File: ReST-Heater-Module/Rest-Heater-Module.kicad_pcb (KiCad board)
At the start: 2 copper layers, 24.5 x 29.5 mm, 35 parts

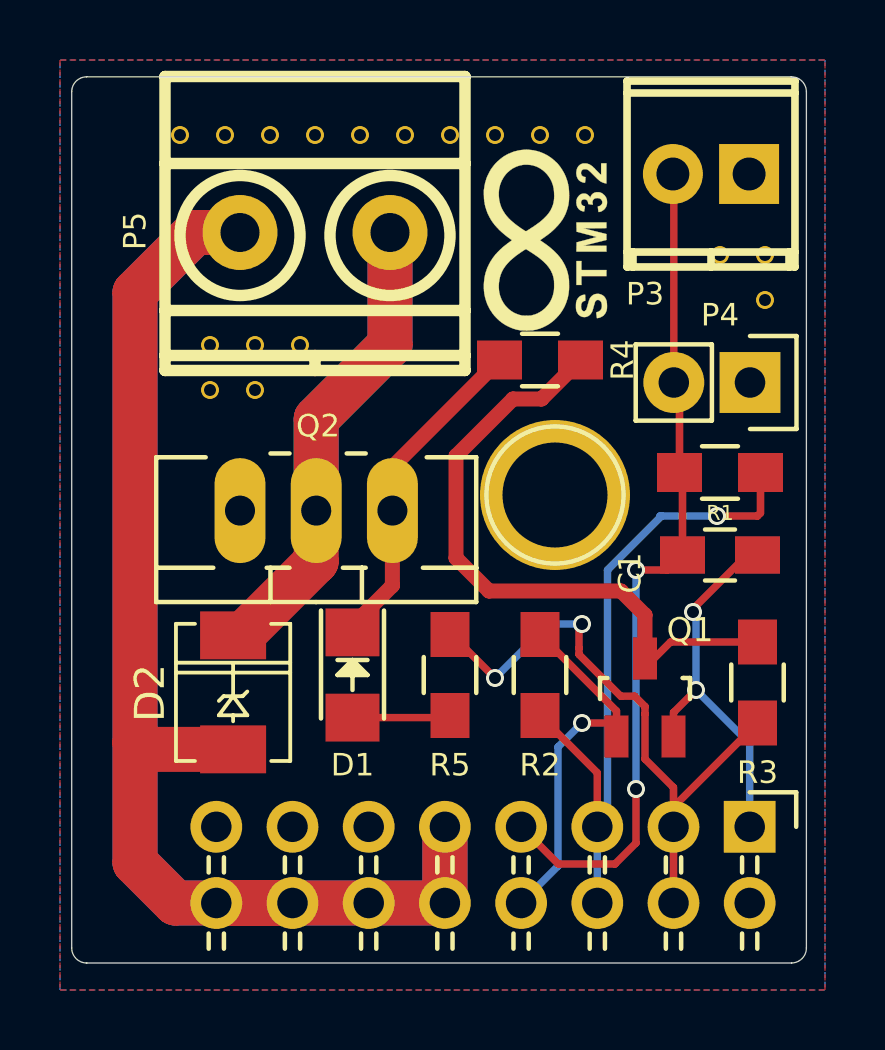
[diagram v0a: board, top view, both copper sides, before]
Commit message: Final release
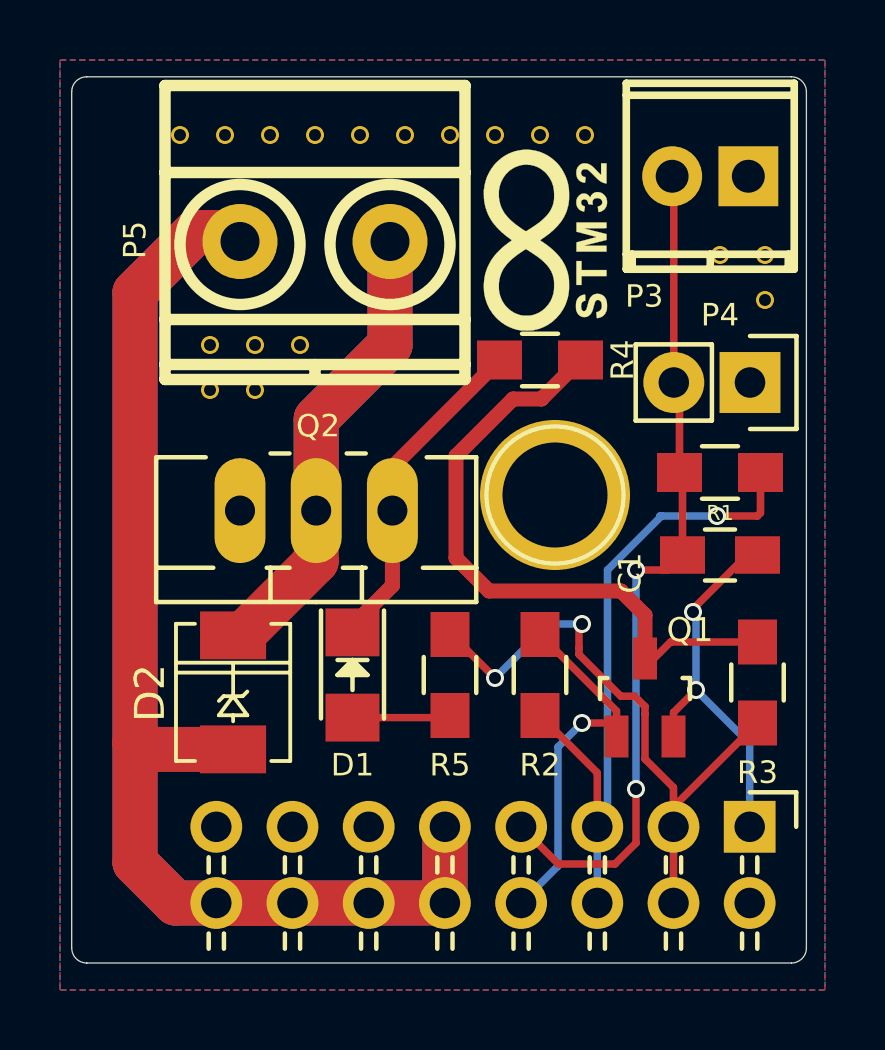
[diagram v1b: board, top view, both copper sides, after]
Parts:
- moved P5 0.30 mm to (141.0, 110.5)
- moved P3 0.08 mm to (154.2, 108.4)
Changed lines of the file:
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@@
     (links 52)
     (no_connects 0)
-    (area 132.5 102.875 159.575 143.485001)
+    (area 132.5 102.875 159.575 135.500001)
     (thickness 1.6)
     (drawings 9)
@@
     (visible_elements 7FFFFFFF)
     (pcbplotparams
-      (layerselection 0x00030_80000001)
-      (usegerberextensions false)
+      (layerselection 0x010f0_80000001)
+      (usegerberextensions true)
       (excludeedgelayer true)
       (linewidth 0.100000)
@@
       (psa4output false)
       (plotreference true)
-      (plotvalue true)
+      (plotvalue false)
       (plotinvisibletext false)
       (padsonsilk false)
@@
       (outputformat 1)
       (mirror false)
-      (drillshape 1)
+      (drillshape 0)
       (scaleselection 1)
-      (outputdirectory ""))
+      (outputdirectory ../Gerber/Heater/))
   )
   (net 0 "")
@@
   )
   (module ReST-Library:screw-2,54-2P (layer F.Cu)
-    (at 154.2 108.3)
+    (at 154.175 108.375)
     (descr "2-way 2.54mm pitch terminal block, Phoenix MPT series")
     (fp_text reference P3 (at -2.2 4 180) (layer F.SilkS)
@@
   )
   (module ReST-Library:screw-5-2P (layer F.Cu)
-    (at 141 110.25)
+    (at 141 110.55)
     (descr "2-way 5mm pitch terminal block, Phoenix MKDS series")
     (fp_text reference P5 (at -6 -0.05 90) (layer F.SilkS)
